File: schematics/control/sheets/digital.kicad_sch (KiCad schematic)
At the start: 17 parts, among them U1 Pico, U12 TL072, U3 MCP4822

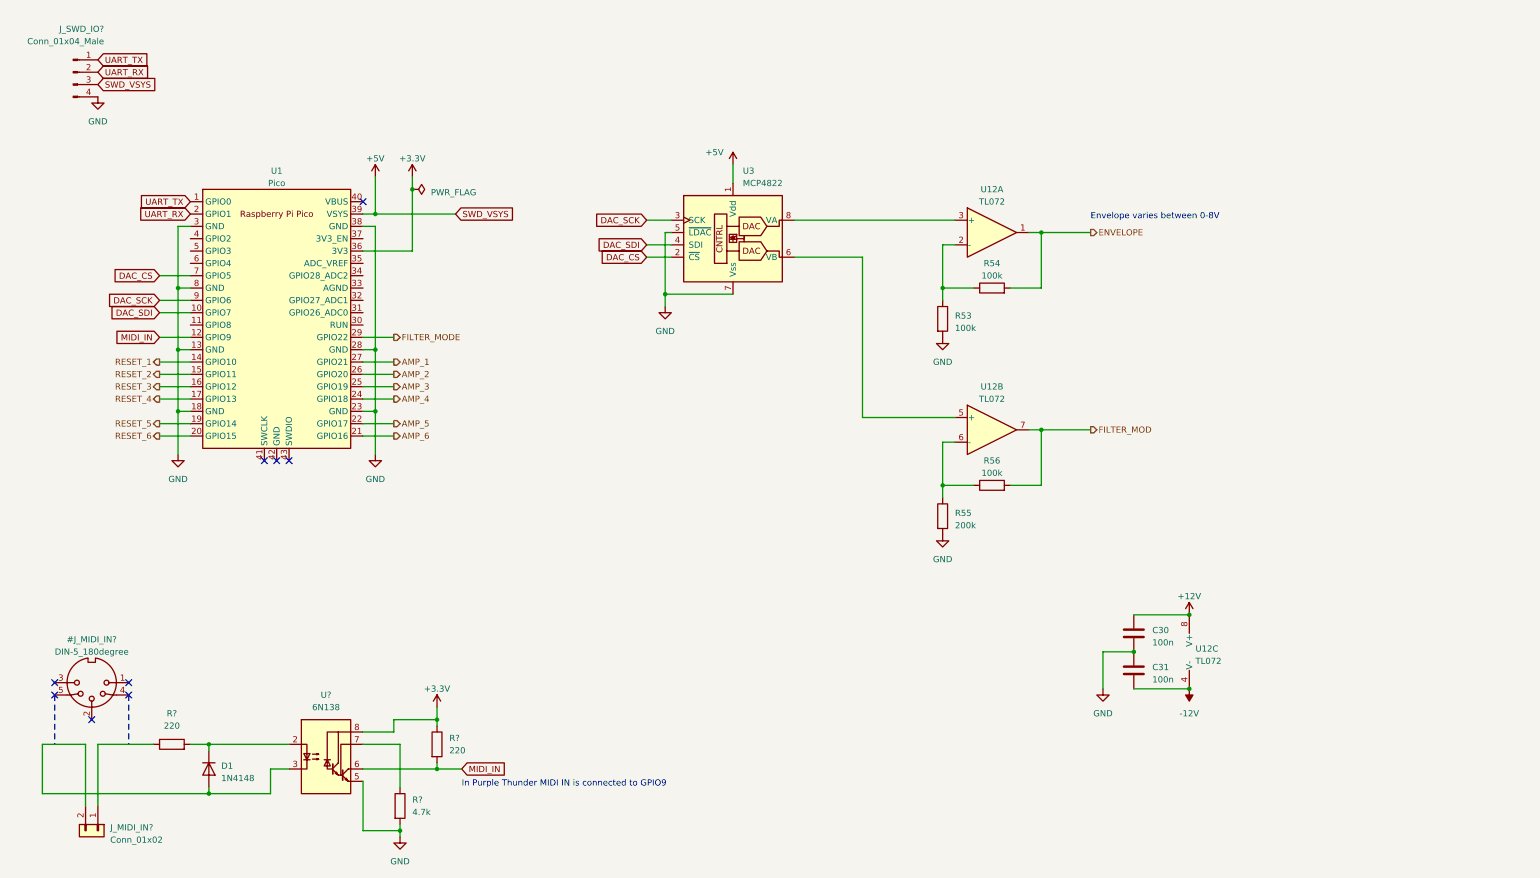
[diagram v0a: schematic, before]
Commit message: Updated VCA
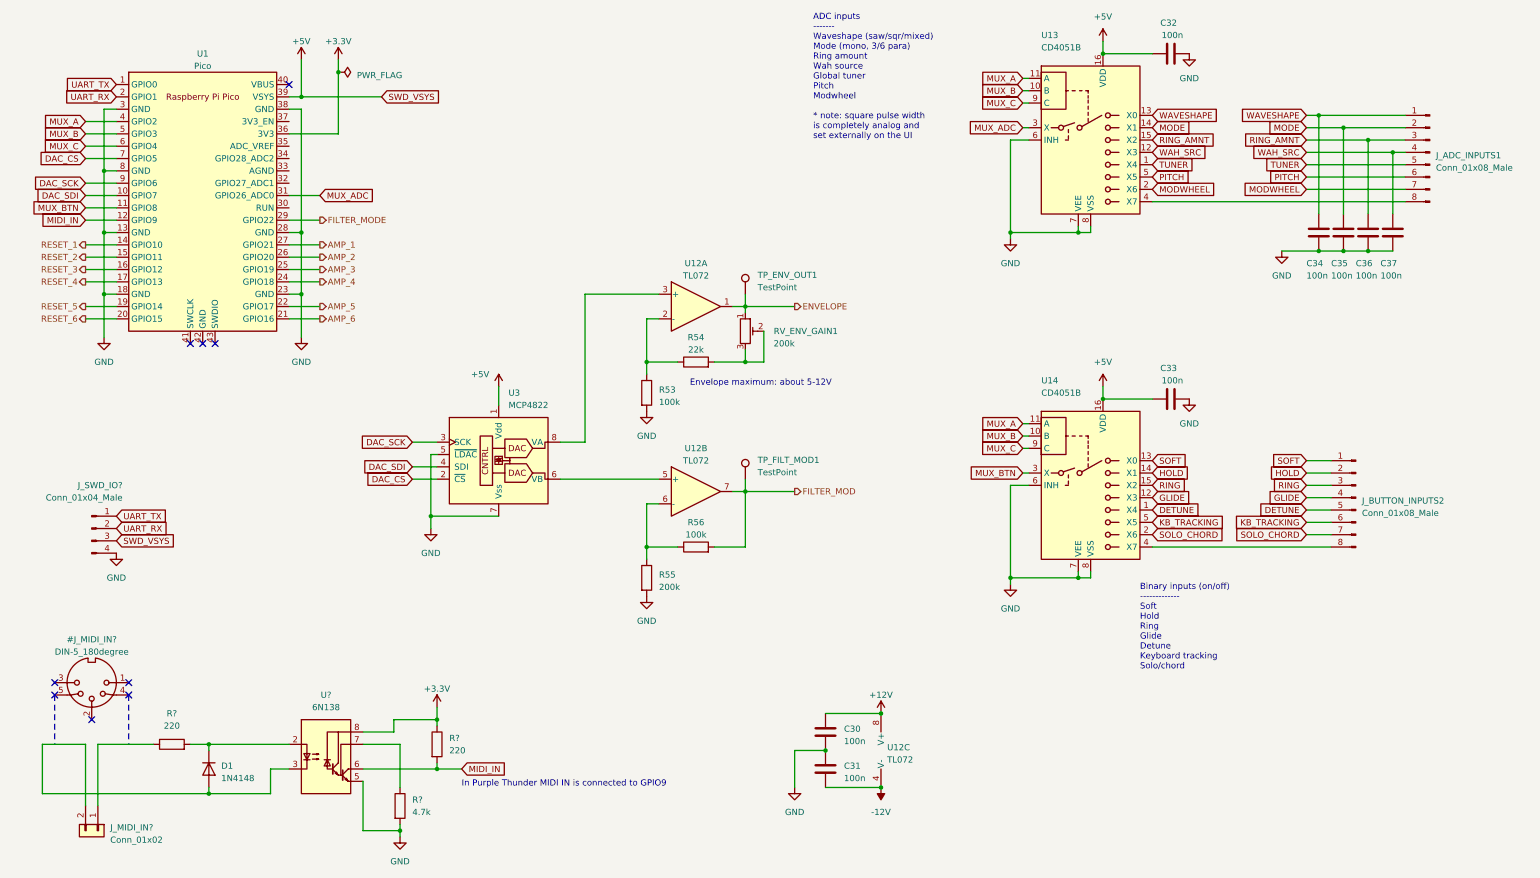
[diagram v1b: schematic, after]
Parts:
- added C32, C33: 100n, Shmoergh_Manual_PCB:C_Disc_D5.0mm_W2.5mm_P2.50mm, symbol Device:C
- added C34, C35, C36, C37: 100n, symbol Device:C
- added J_ADC_INPUTS1, J_BUTTON_INPUTS2: Conn_01x08_Male, Shmoergh_Manual_PCB:NSL25_01x08_Vertical, symbol Connector:Conn_01x08_Male
- added RV_ENV_GAIN1: 200k, symbol Device:R_Potentiometer_Trim
- added TP_ENV_OUT1, TP_FILT_MOD1: TestPoint, symbol Connector:TestPoint
- added U13, U14: CD4051B, Shmoergh_Manual_PCB:DIP-16_W7.62mm, symbol Analog_Switch:CD4051B
- R54: value 100k -> 22k
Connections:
- net +5V: now also C32.1, C33.1, U13.16 (VDD), U14.16 (VDD)
- net ENVELOPE: now also RV_ENV_GAIN1.1, TP_ENV_OUT1.1; no longer R54.2
- net FILTER_MOD: now also TP_FILT_MOD1.1
- net GND: now also C32.2, C33.2, C34.2, C35.2, C36.2, C37.2, U13.6 (INH), U13.7 (VEE), U13.8 (VSS), U14.6 (INH), U14.7 (VEE), U14.8 (VSS)
- net MUX_BTN: now reaches U1.11 (GPIO8)
- net MUX_BTN: now also U14.3 (X)
- net MUX_ADC: now reaches U1.31 (GPIO26_ADC0)
- net MUX_ADC: now also U13.3 (X)
- net MUX_A: now reaches U1.4 (GPIO2)
- net MUX_A: now also U13.11 (A), U14.11 (A)
- net MUX_B: now reaches U1.5 (GPIO3)
- net MUX_B: now also U13.10 (B), U14.10 (B)
- net MUX_C: now reaches U1.6 (GPIO4)
- net MUX_C: now also U13.9 (C), U14.9 (C)
- new net: R54.2, RV_ENV_GAIN1.2, RV_ENV_GAIN1.3
- new net: J_ADC_INPUTS1.8 (Pin_8), U13.4 (X7)
- new net: J_BUTTON_INPUTS2.8 (Pin_8), U14.4 (X7)
- new net DETUNE: J_BUTTON_INPUTS2.5 (Pin_5), U14.1 (X4)
- new net GLIDE: J_BUTTON_INPUTS2.4 (Pin_4), U14.12 (X3)
- new net HOLD: J_BUTTON_INPUTS2.2 (Pin_2), U14.14 (X1)
- new net KB_TRACKING: J_BUTTON_INPUTS2.6 (Pin_6), U14.5 (X5)
- new net MODE: C35.1, J_ADC_INPUTS1.2 (Pin_2), U13.14 (X1)
- new net MODWHEEL: J_ADC_INPUTS1.7 (Pin_7), U13.2 (X6)
- new net PITCH: J_ADC_INPUTS1.6 (Pin_6), U13.5 (X5)
- new net RING: J_BUTTON_INPUTS2.3 (Pin_3), U14.15 (X2)
- new net RING_AMNT: C36.1, J_ADC_INPUTS1.3 (Pin_3), U13.15 (X2)
- new net SOFT: J_BUTTON_INPUTS2.1 (Pin_1), U14.13 (X0)
- new net SOLO_CHORD: J_BUTTON_INPUTS2.7 (Pin_7), U14.2 (X6)
- new net TUNER: J_ADC_INPUTS1.5 (Pin_5), U13.1 (X4)
- new net WAH_SRC: C37.1, J_ADC_INPUTS1.4 (Pin_4), U13.12 (X3)
- new net WAVESHAPE: C34.1, J_ADC_INPUTS1.1 (Pin_1), U13.13 (X0)
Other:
- note added: "ADC inputs ------- Waveshape (saw/sqr/mixed) Mode (mono, 3/6 para) Ring amount Wah source Global tuner Pitch Modwheel * note: square pulse width is completely analog and set externally on the UI"
- note added: "Binary inputs (on/off) ------------- Soft Hold Ring Glide Detune Keyboard tracking Solo/chord"
- note added: "Envelope maximum: about 5-12V"
- note removed: "Envelope varies between 0-8V"
- moved on the sheet: C30, C31, J_SWD_IO?, R53, R54, R55, R56, U1, U12A, U12B, U12C, U3
